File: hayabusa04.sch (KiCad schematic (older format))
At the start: 24 parts, among them SW1 SW_Push, U1 ATmega32U4-AU, Y1 16MHz

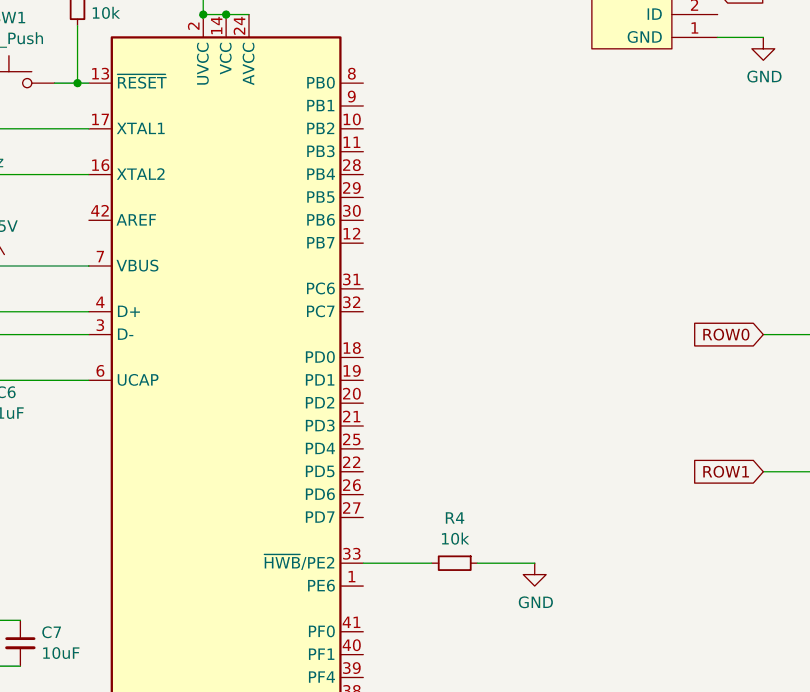
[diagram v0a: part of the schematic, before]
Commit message: updated pcb
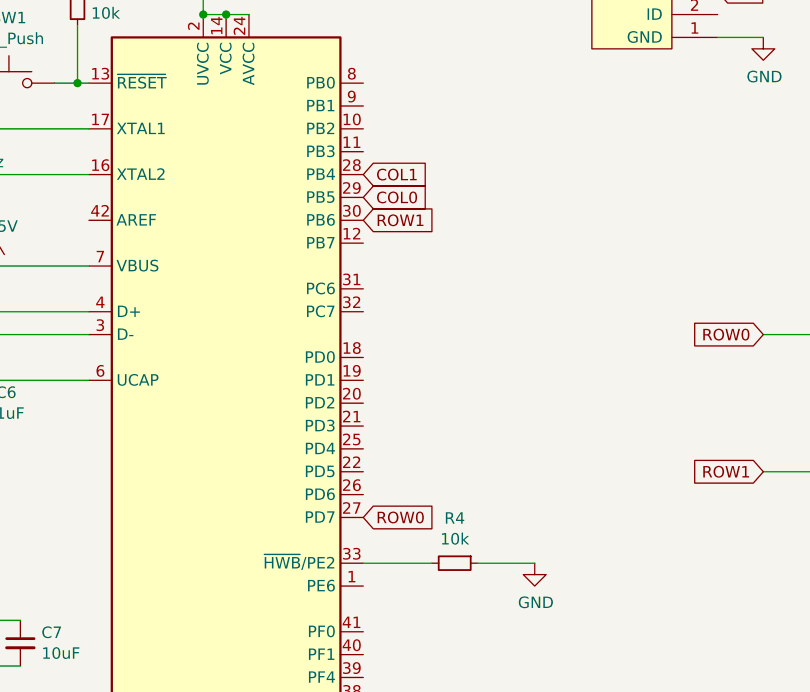
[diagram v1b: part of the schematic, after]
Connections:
- net COL0: now also U1.29 (PB5)
- net COL1: now also U1.28 (PB4)
- net ROW0: now also U1.27 (PD7)
- net ROW1: now also U1.30 (PB6)
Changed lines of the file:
@@
 Text GLabel 5400 4000 0    50   Input ~ 0
 ROW1
+Text GLabel 3650 2700 2    50   Input ~ 0
+COL1
+Text GLabel 3650 2800 2    50   Input ~ 0
+COL0
+Text GLabel 3650 2900 2    50   Input ~ 0
+ROW1
+Text GLabel 3650 4200 2    50   Input ~ 0
+ROW0
 $EndSCHEMATC
